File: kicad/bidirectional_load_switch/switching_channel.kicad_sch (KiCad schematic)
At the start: 14 parts, among them U201 SN74LVC1G17DCKR, U202 UCC23313DWYR, U203 SISS94DN-T1-GE3, U204 SISS94DN-T1-GE3

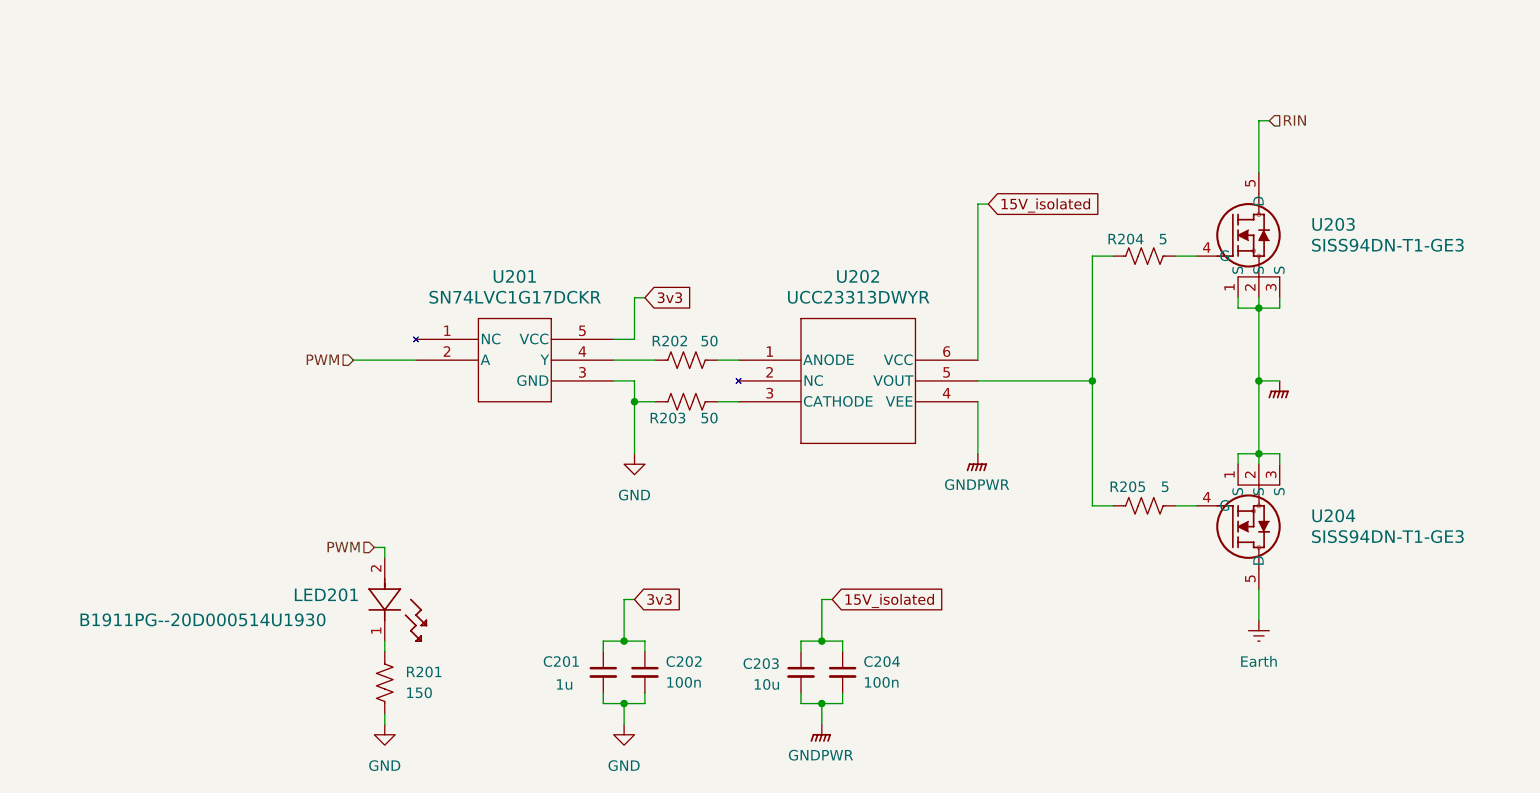
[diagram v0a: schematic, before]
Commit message: load switch
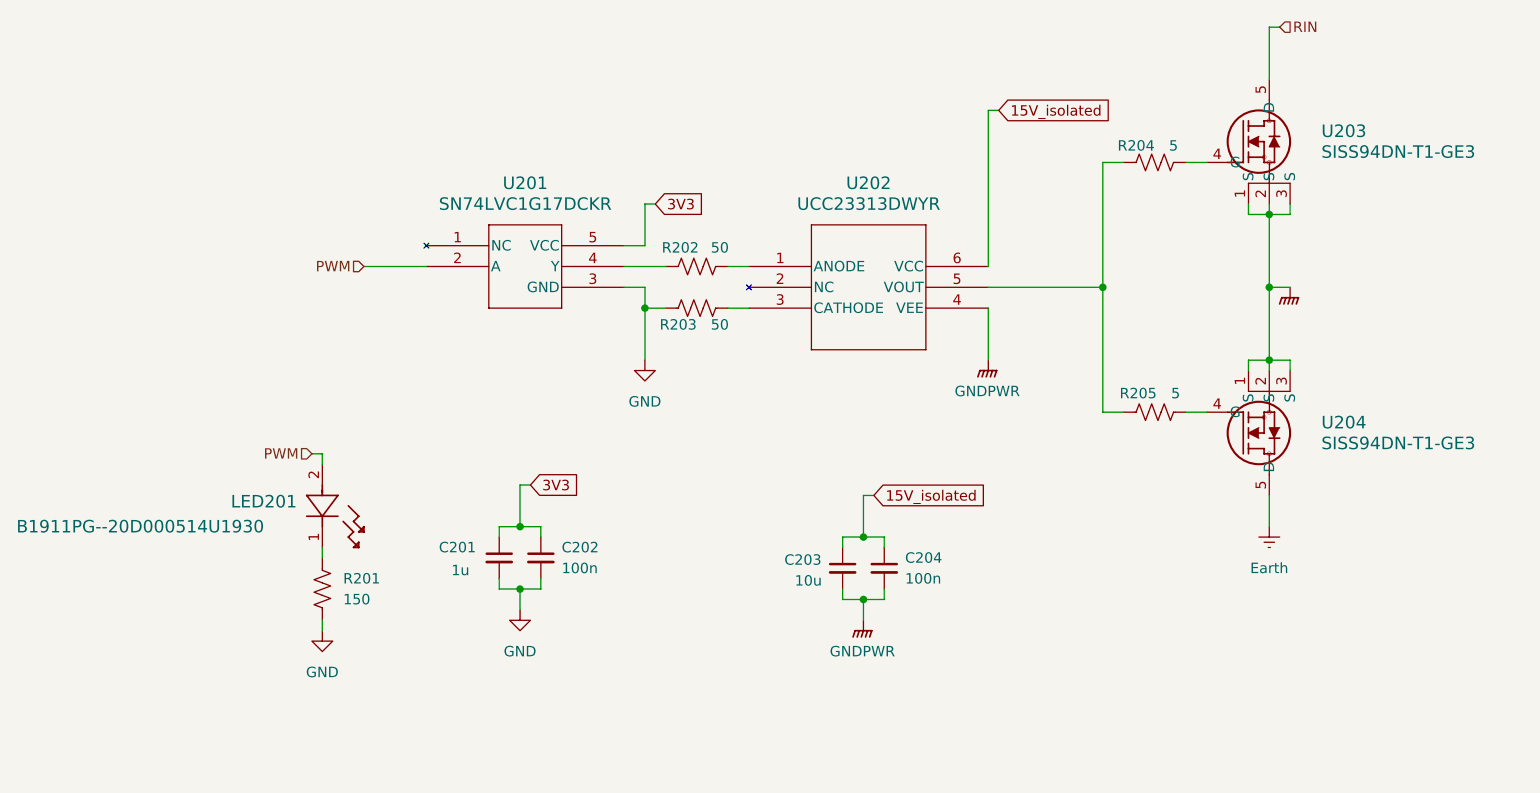
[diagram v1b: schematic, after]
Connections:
- net 3v3 renamed 3V3
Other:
- moved on the sheet: C201, C202, C203, C204, LED201, R201, R202, R203, R204, R205, U201, U202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
